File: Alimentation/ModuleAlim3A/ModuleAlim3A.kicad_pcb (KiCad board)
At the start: 2 copper layers, 40 x 42.8 mm, 12 parts, among them J1 Inhibit, J2 Alim. IN / OUT, U1 PTN78060W_EUW-7

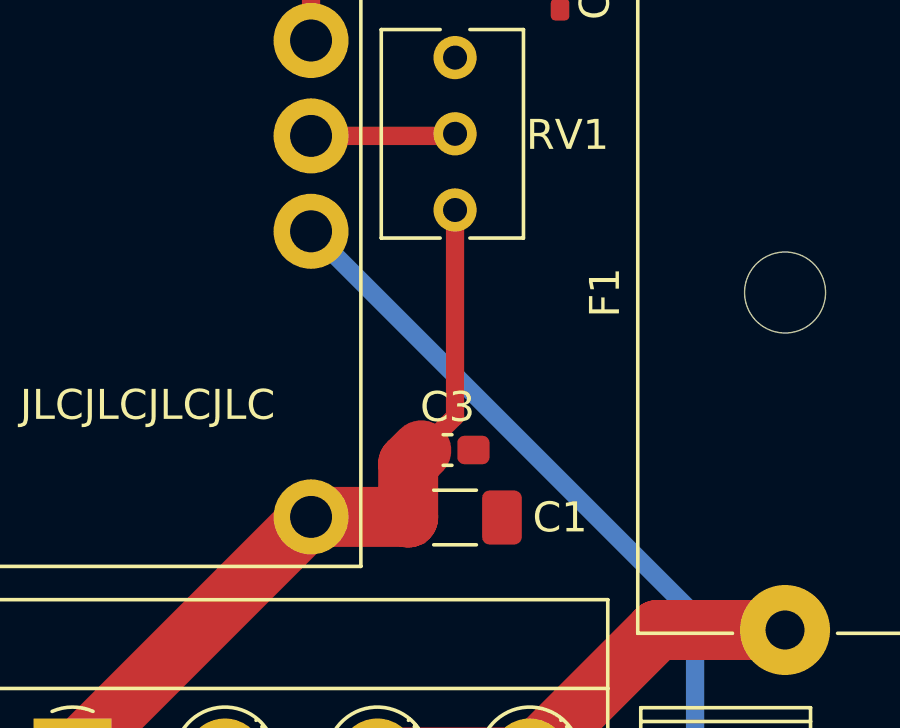
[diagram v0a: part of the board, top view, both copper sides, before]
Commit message: Finalisation pour commande pack Alimentation 14/02/2021
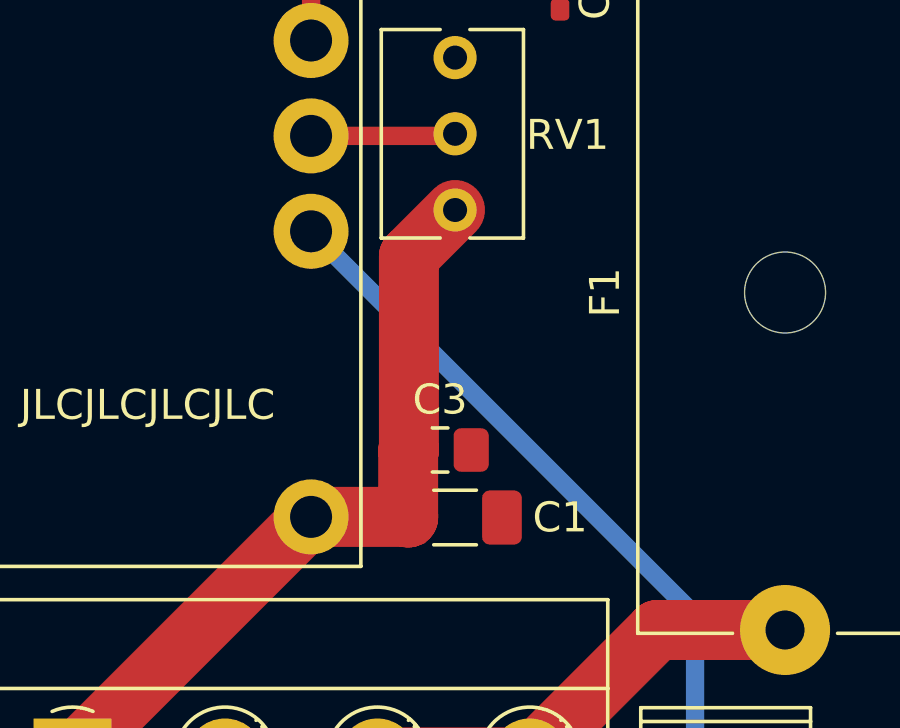
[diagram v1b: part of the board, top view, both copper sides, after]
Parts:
- C3: footprint Capacitor_SMD:C_0603_1608Metric_Pad1.08x0.95mm_HandSolder -> Capacitor_SMD:C_0805_2012Metric_Pad1.18x1.45mm_HandSolder
- moved C3 0.25 mm to (148.0, 75.8)
